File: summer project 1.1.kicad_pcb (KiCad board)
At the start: 2 copper layers, 47.4 x 23.2 mm, 11 parts, among them J1 Conn_01x02_Socket, J2 Conn_01x02_Socket, J3 Screw_Terminal_01x02, Q1 NMOS, Q2 NMOS, U1 LM5050-1_mod2, U2 LM5050-1_mod2

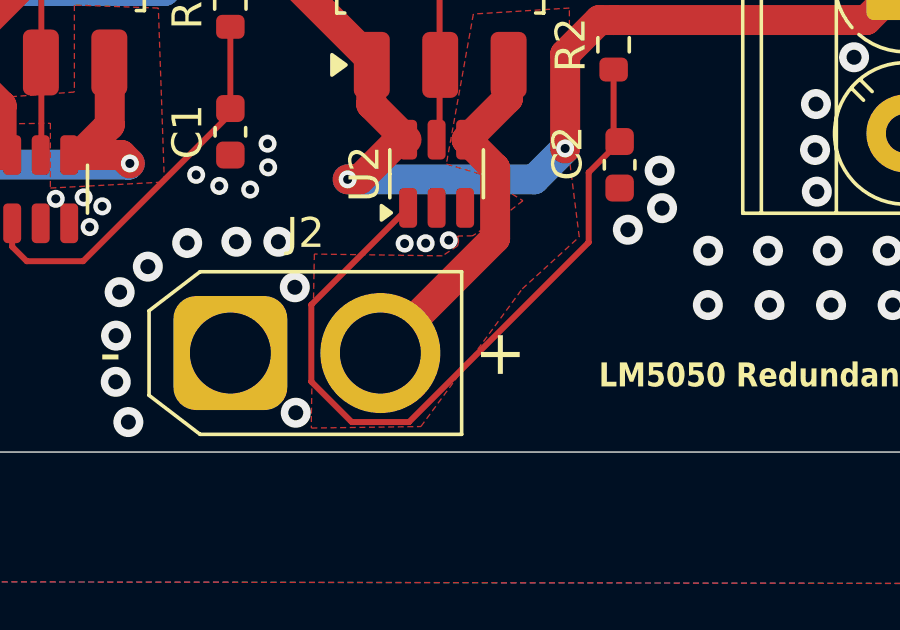
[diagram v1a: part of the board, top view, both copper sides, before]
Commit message: final commit
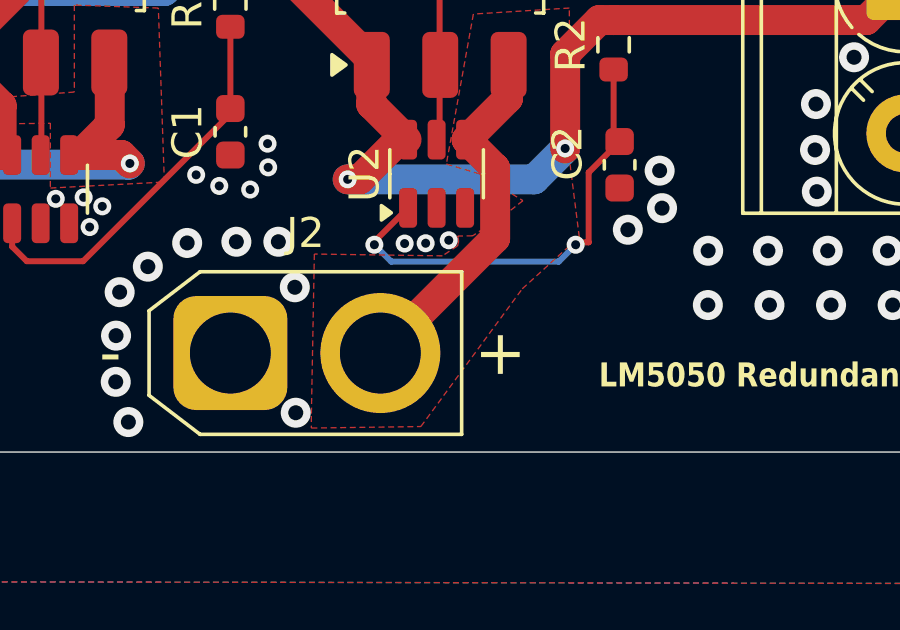
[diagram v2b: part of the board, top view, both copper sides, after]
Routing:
- net Net-(U2-VS): track 25.7 -> 15.6 mm, vias 0 -> 2
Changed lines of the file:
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@@
 	)
 	(segment
-		(start 149.464 88.230106)
-		(end 143.473106 94.221)
-		(width 0.2)
-		(layer "F.Cu")
-		(net 7)
-	)
-	(segment
-		(start 140.219 90.3085)
-		(end 143.445 87.0825)
-		(width 0.2)
-		(layer "F.Cu")
-		(net 7)
-	)
-	(segment
-		(start 141.566894 94.221)
-		(end 140.219 92.873106)
-		(width 0.2)
-		(layer "F.Cu")
-		(net 7)
-	)
-	(segment
-		(start 140.219 92.873106)
-		(end 140.219 90.3085)
+		(start 142.32 88.31)
+		(end 142.32 88.2075)
 		(width 0.2)
 		(layer "F.Cu")
@@
 	)
 	(segment
-		(start 143.473106 94.221)
-		(end 141.566894 94.221)
+		(start 142.32 88.2075)
+		(end 143.445 87.0825)
+		(width 0.2)
+		(layer "F.Cu")
+		(net 7)
+	)
+	(segment
+		(start 149.464 88.230106)
+		(end 149.109894 88.230106)
 		(width 0.2)
 		(layer "F.Cu")
@@
 		(net 7)
 	)
+	(segment
+		(start 149.109894 88.230106)
+		(end 149.03 88.31)
+		(width 0.2)
+		(layer "F.Cu")
+		(net 7)
+	)
+	(via
+		(at 142.32 88.31)
+		(size 0.6)
+		(drill 0.3)
+		(layers "F.Cu" "B.Cu")
+		(net 7)
+	)
+	(via
+		(at 149.03 88.31)
+		(size 0.6)
+		(drill 0.3)
+		(layers "F.Cu" "B.Cu")
+		(net 7)
+	)
+	(segment
+		(start 142.881 88.871)
+		(end 142.32 88.31)
+		(width 0.2)
+		(layer "B.Cu")
+		(net 7)
+	)
+	(segment
+		(start 148.469 88.871)
+		(end 142.881 88.871)
+		(width 0.2)
+		(layer "B.Cu")
+		(net 7)
+	)
+	(segment
+		(start 149.03 88.31)
+		(end 148.469 88.871)
+		(width 0.2)
+		(layer "B.Cu")
+		(net 7)
+	)
